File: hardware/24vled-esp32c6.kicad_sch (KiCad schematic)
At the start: 5 parts, among them J1 Conn_01x20, J2 Conn_01x20, J3 Barrel_Jack, J5 2604-1106, U1 LM2596S-5

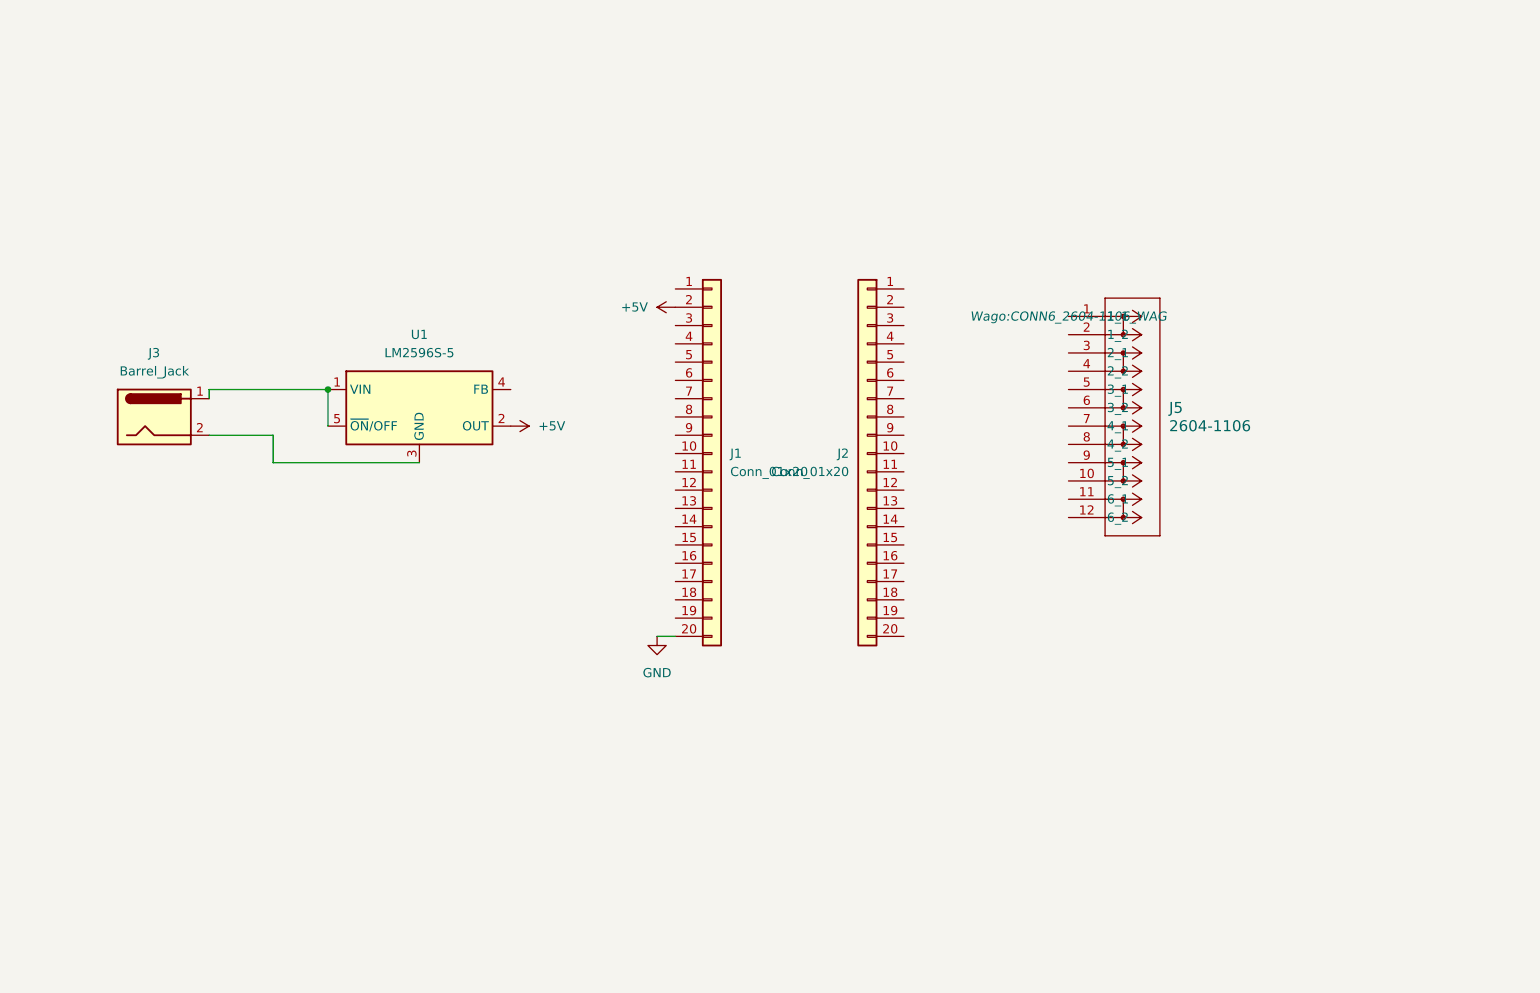
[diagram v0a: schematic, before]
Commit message: hardware v1
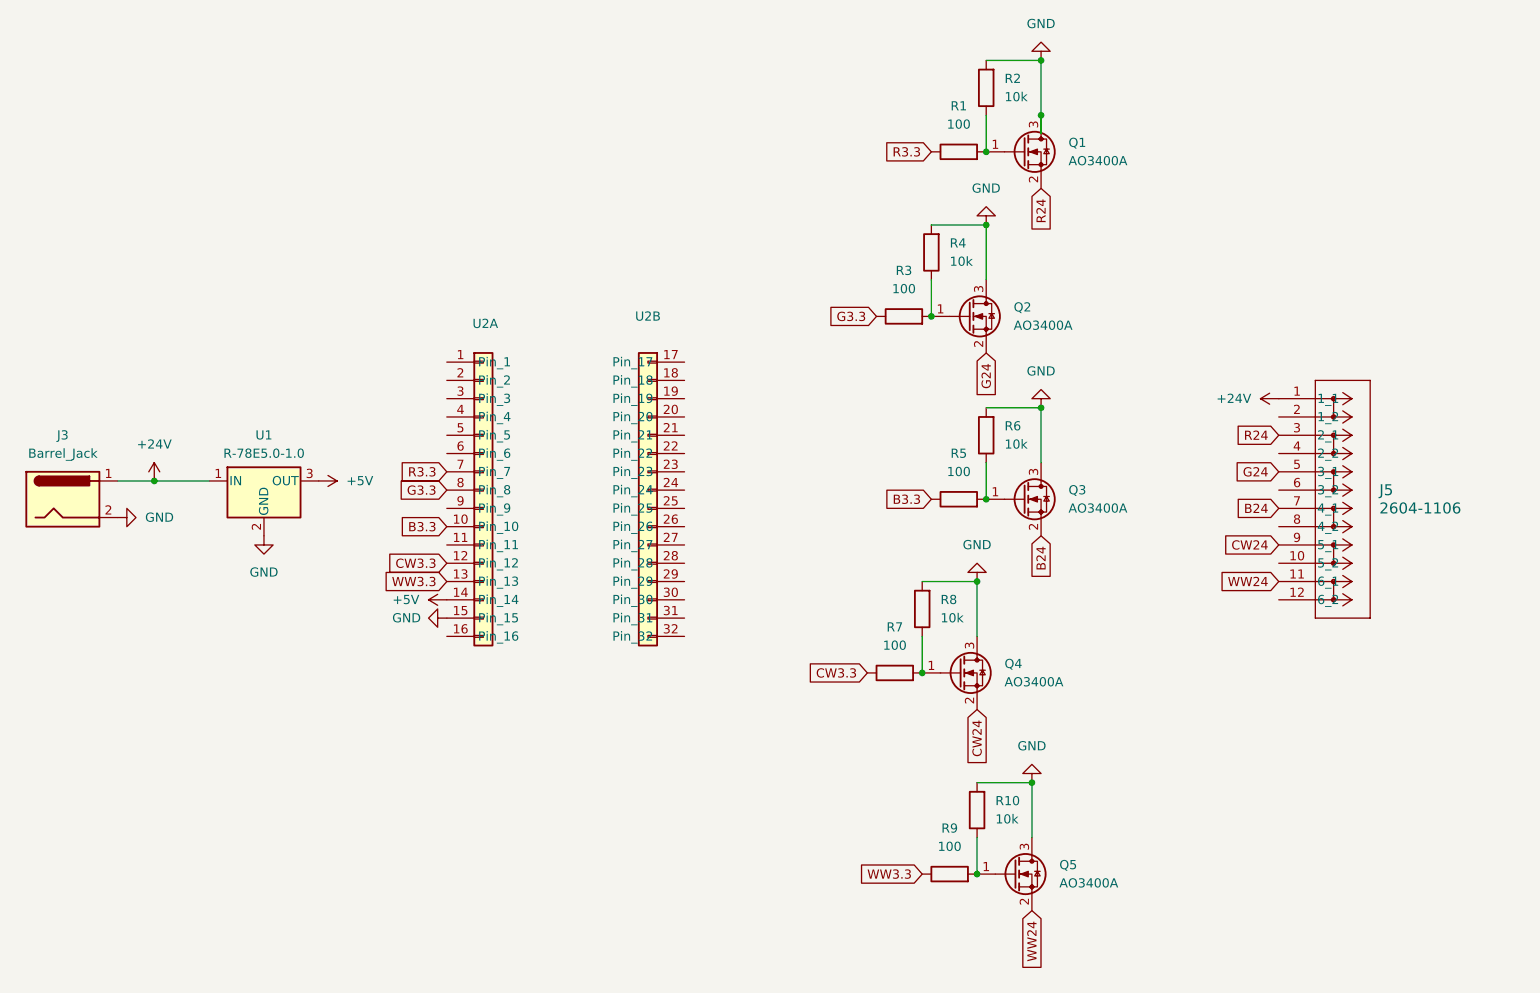
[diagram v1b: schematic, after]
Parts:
- removed J1, J2: Conn_01x20, Connector_PinHeader_2.54mm:PinHeader_1x20_P2.54mm_Vertical, symbol Connector_Generic:Conn_01x20
- removed U1: LM2596S-5, Package_TO_SOT_SMD:TO-263-5_TabPin3, symbol Regulator_Switching:LM2596S-5
- added Q1, Q2, Q3, Q4, Q5: AO3400A, Package_TO_SOT_SMD:SOT-23, symbol Transistor_FET:AO3400A
- added R1, R3, R5, R7, R9: 100, Resistor_SMD:R_0201_0603Metric, symbol Device:R
- added R10, R2, R4, R6, R8: 10k, Resistor_SMD:R_0201_0603Metric, symbol Device:R
- added U1: R-78E5.0-1.0, Converter_DCDC:Converter_DCDC_RECOM_R-78E-0.5_THT, symbol Regulator_Switching:R-78E5.0-1.0
- added U2: ~, Library:Waveshare ESP32c6, symbol Symbols:Waveshare_ESP32c6
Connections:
- net +5V: now also U1.3 (OUT), U2.14 (Pin_14)
- net GND: now also J3.2, Q1.3 (D), Q2.3 (D), Q3.3 (D), Q4.3 (D), Q5.3 (D), R10.2, R2.2, R4.2, R6.2, R8.2, U1.2 (GND), U2.15 (Pin_15)
- net +24V: now reaches J5.1 (1_1)
- net +24V: now also J3.1, U1.1 (IN)
- net WW24: now reaches J5.11 (6_1)
- net WW24: now also Q5.2 (S)
- net R24: now reaches J5.3 (2_1)
- net R24: now also Q1.2 (S)
- net G24: now reaches J5.5 (3_1)
- net G24: now also Q2.2 (S)
- net B24: now reaches J5.7 (4_1)
- net B24: now also Q3.2 (S)
- net CW24: now reaches J5.9 (5_1)
- net CW24: now also Q4.2 (S)
- new net: Q2.1 (G), R3.2, R4.1
- new net: Q3.1 (G), R5.2, R6.1
- new net: Q5.1 (G), R10.1, R9.2
- new net: Q1.1 (G), R1.2, R2.1
- new net: Q4.1 (G), R7.2, R8.1
- new net B3.3: R5.1, U2.10 (Pin_10)
- new net CW3.3: R7.1, U2.12 (Pin_12)
- new net G3.3: R3.1, U2.8 (Pin_8)
- new net R3.3: R1.1, U2.7 (Pin_7)
- new net WW3.3: R9.1, U2.13 (Pin_13)
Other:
- moved on the sheet: J3, J5

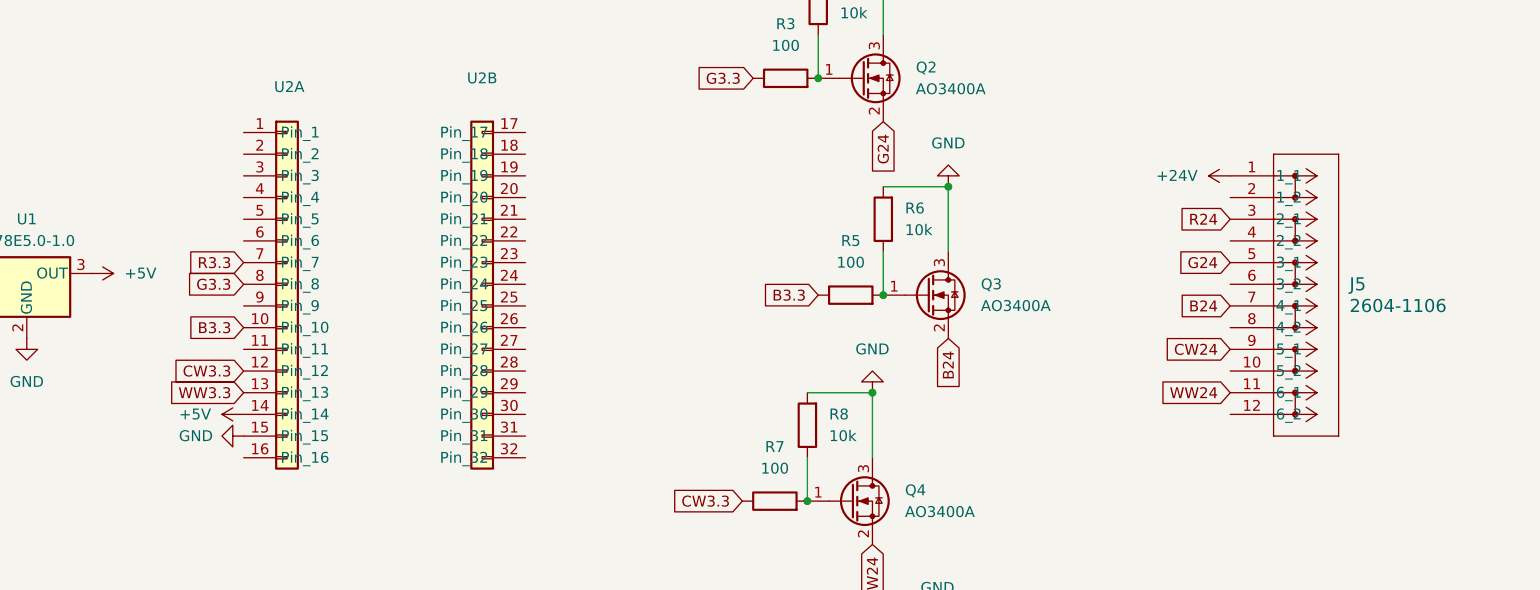
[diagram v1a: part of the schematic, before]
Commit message: hardware v2
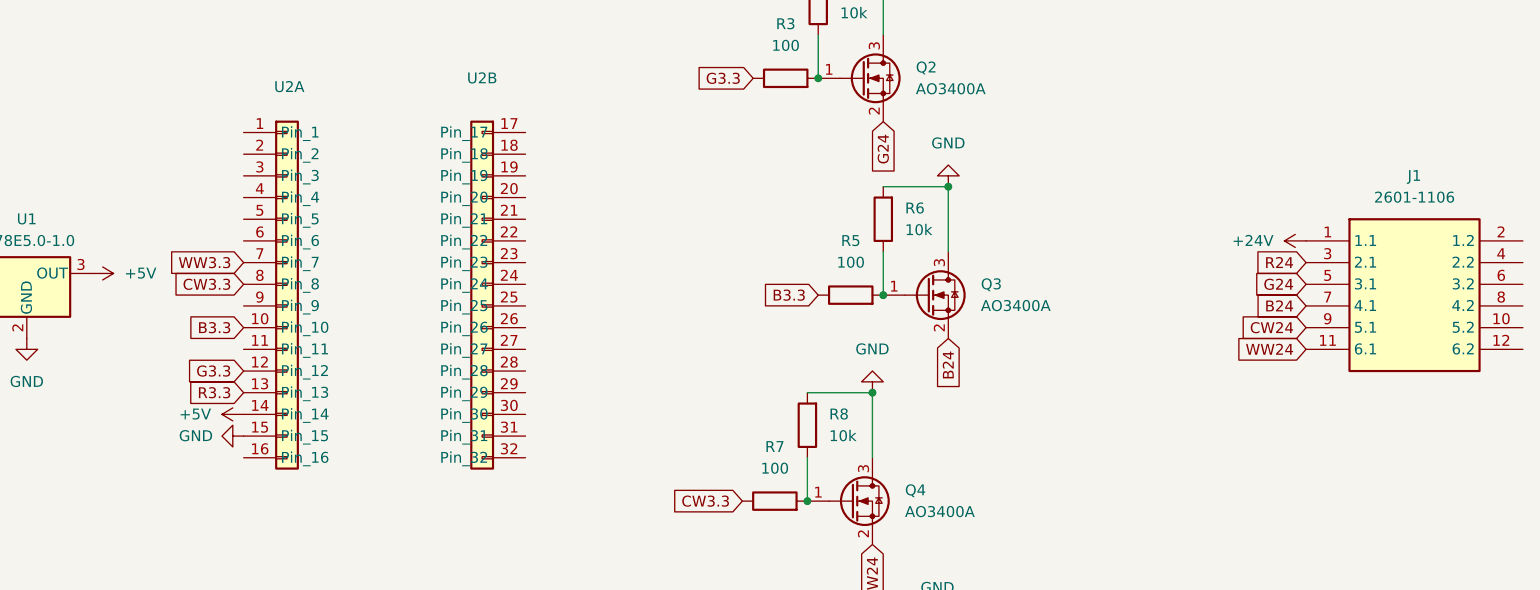
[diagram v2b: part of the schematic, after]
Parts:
- removed J5: 2604-1106, Wago:CONN6_2604-1106_WAG, symbol Wago:2604-1106
- added J1: 2601-1106, External:26011106, symbol External:2601-1106
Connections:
- net +24V: now also J1.1 (1.1)
- net B24: now also J1.7 (4.1)
- net CW24: now also J1.9 (5.1)
- net CW3.3: now also U2.8 (Pin_8); no longer U2.12 (Pin_12)
- net G24: now also J1.5 (3.1)
- net G3.3: now also U2.12 (Pin_12); no longer U2.8 (Pin_8)
- net R24: now also J1.3 (2.1)
- net R3.3: now also U2.13 (Pin_13); no longer U2.7 (Pin_7)
- net WW24: now also J1.11 (6.1)
- net WW3.3: now also U2.7 (Pin_7); no longer U2.13 (Pin_13)
